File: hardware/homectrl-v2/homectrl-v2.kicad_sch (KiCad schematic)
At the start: 127 parts, among them J1 Barrel_Jack, J2 PUMP1_CONN, J3 PUMP2_CONN, J4 STEP_CONN, J5 USB_C_CONN, J6 SMS1_CONN, J7 ALS_CONN, J8 FSW1_CONN, Q1 AO3407A, Q2 2N7002, Q3 ZXMN3A01ZTA, Q4 ZXMN3A01ZTA, Q5 AO3400A, SW1 S3_RESET_SW, SW2 S3_BOOT_SW, U1 TPS5405DR, U2 MCP1826S, U3 DMP4065S-7, U4 ESP32-S3-WROOM-1, U5 TMC2209, U7 TPD4E001DRLR, U8 TPD2E001DRLR, U9 SI2347DS-T1-GE3

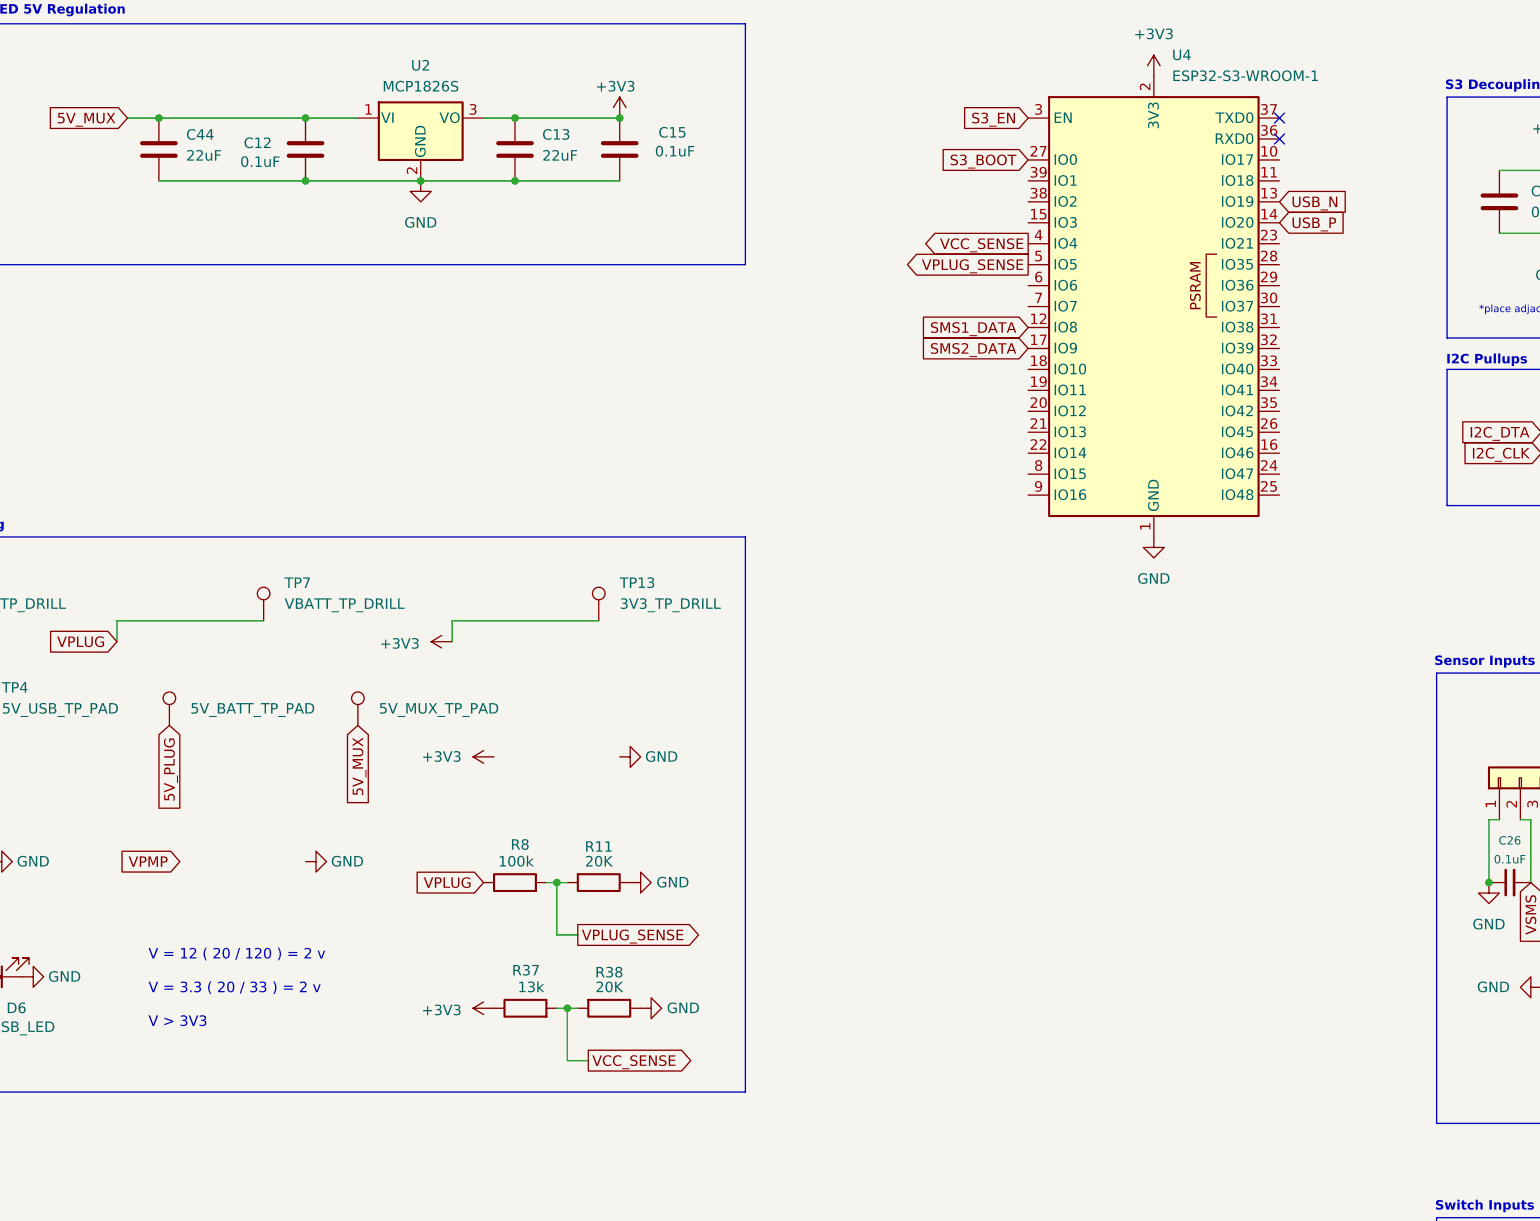
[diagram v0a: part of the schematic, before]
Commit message: misc work
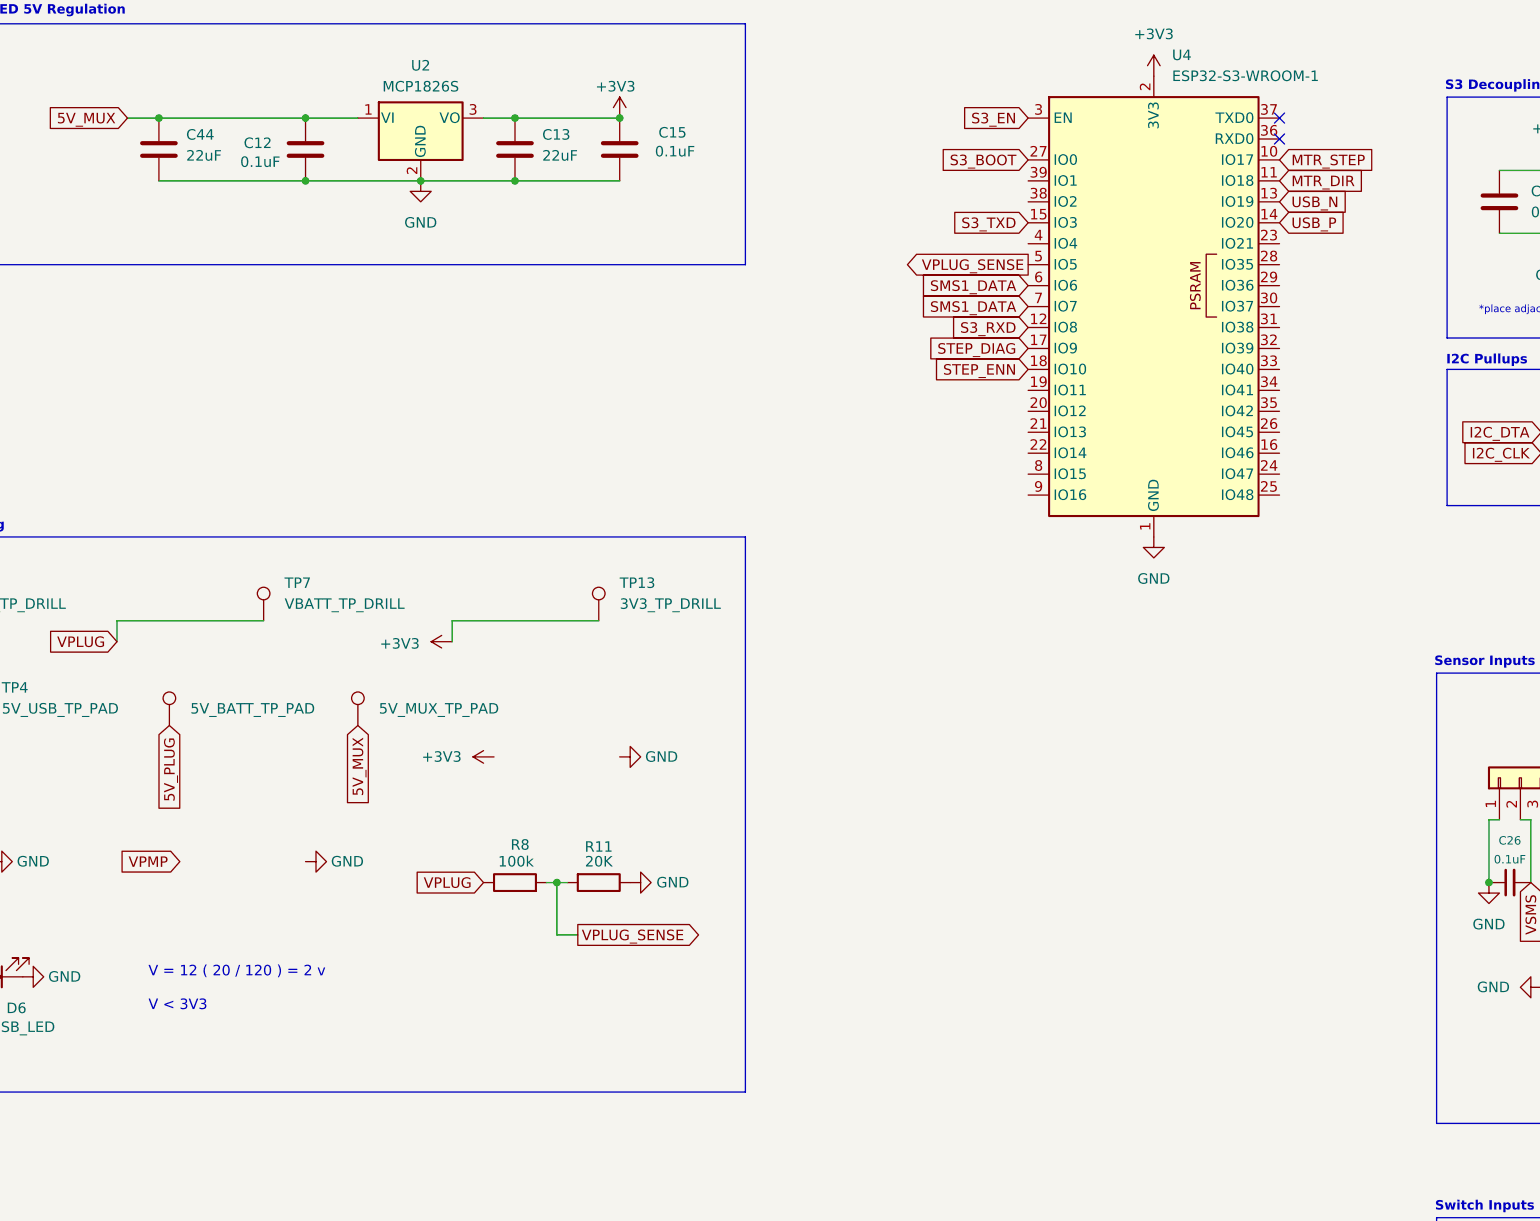
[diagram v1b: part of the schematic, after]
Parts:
- removed R37: 13k, Resistor_SMD:R_0402_1005Metric, symbol Device:R
- removed R38: 20K, Resistor_SMD:R_0402_1005Metric, symbol Device:R
- Q3, Q4: footprint ZXMN3_DIO -> Package_TO_SOT_SMD:SOT-89-3
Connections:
- net MTR_DIR: now also U4.11 (IO18)
- net MTR_STEP: now also U4.10 (IO17)
- net S3_RXD: now also U4.12 (IO8)
- net S3_TXD: now also U4.15 (IO3)
- net SMS1_DATA: now also U4.6 (IO6), U4.7 (IO7); no longer U4.12 (IO8)
- net SMS2_DATA: no longer U4.17 (IO9)
- net STEP_DIAG: now also U4.17 (IO9)
- net STEP_ENN: now also U4.18 (IO10)
- net VCC_SENSE: no longer names the net of U4.4 (IO4)
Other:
- note added: "V = 12 ( 20 / 120 ) = 2 v V < 3V3"
- note removed: "V = 12 ( 20 / 120 ) = 2 v V = 3.3 ( 20 / 33 ) = 2 v V > 3V3"
